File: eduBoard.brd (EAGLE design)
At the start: 101.6 x 80 mm, 31 parts, among them CN1 LED-RGB1, CN2 LED-RGB2, CN3 LED-RGB3

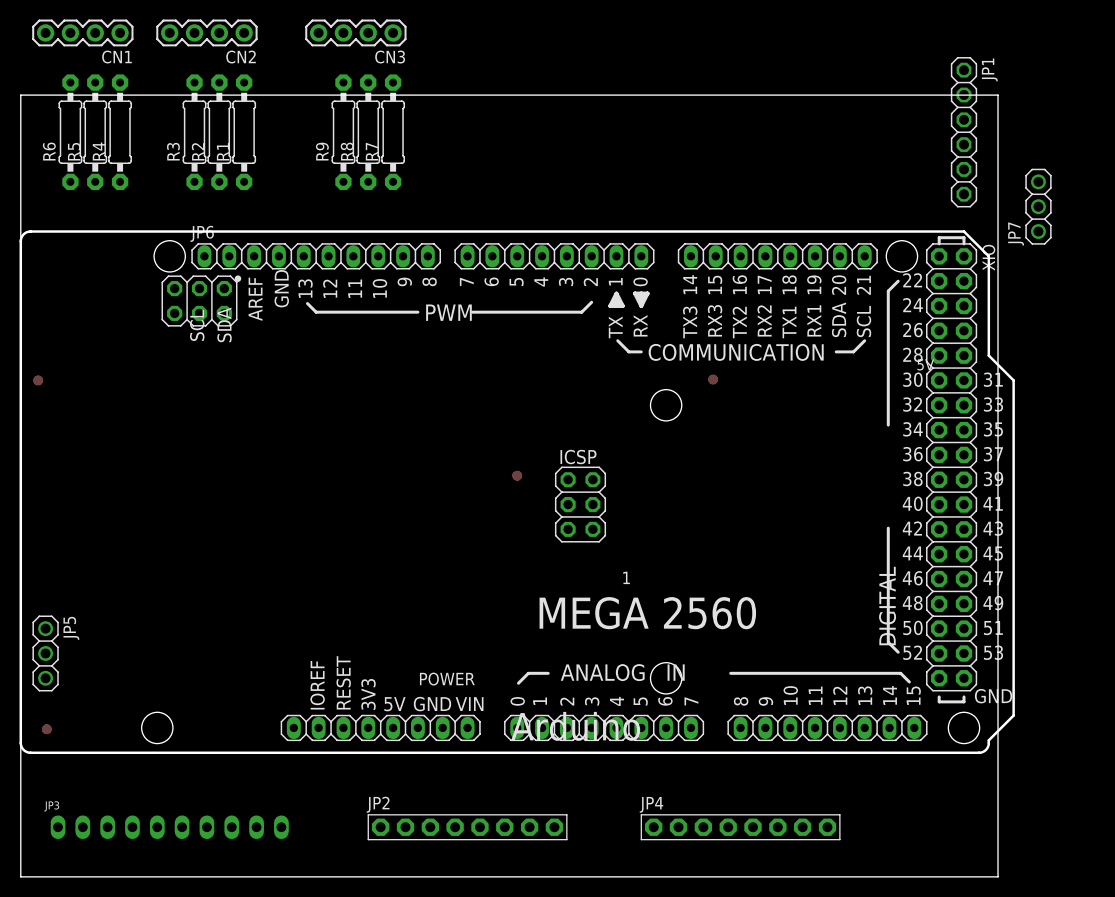
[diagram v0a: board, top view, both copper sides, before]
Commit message: updates, ready for beutification
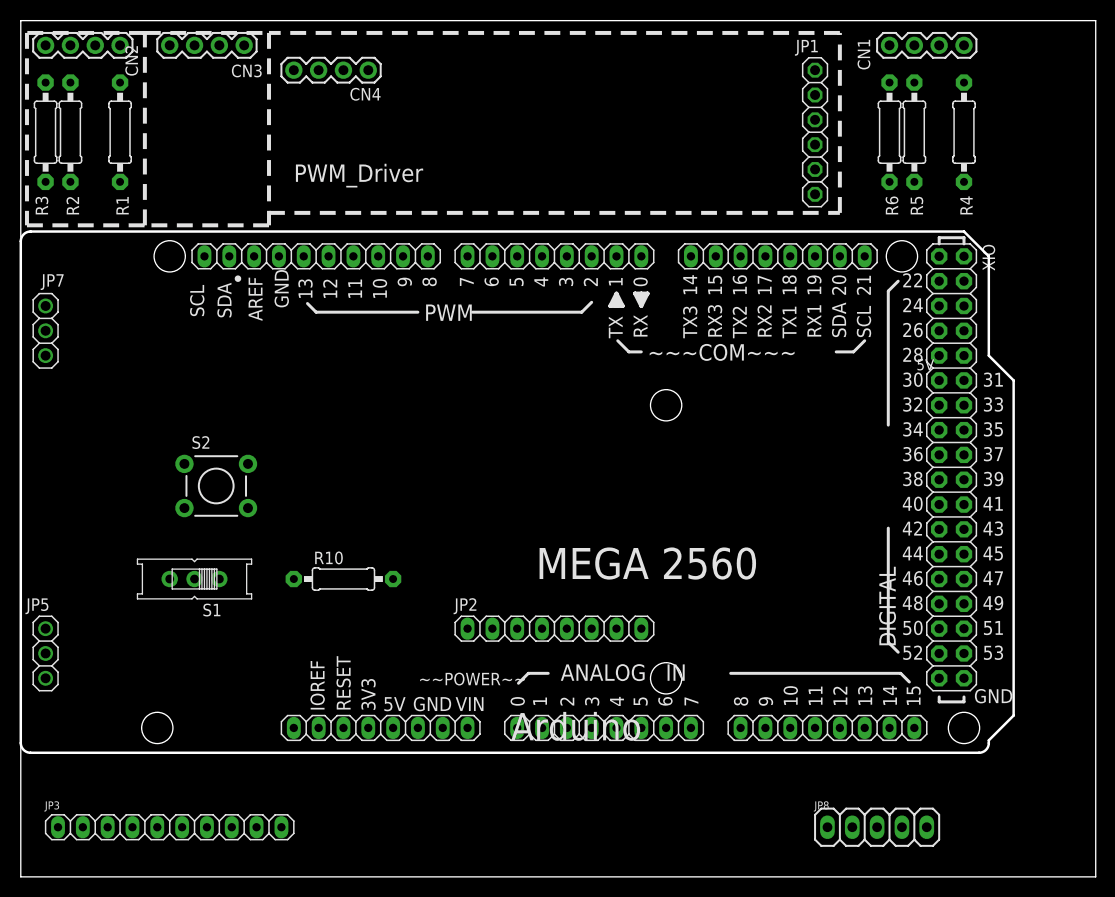
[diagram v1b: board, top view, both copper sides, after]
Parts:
- removed FD1, FD2, FD3, FD4: FIDUCIALMOUNT, SmartPrj:FIDUCIA-MOUNT
- removed ICSP, ICSP1: 3x2M, SmartPrj:2X03
- removed JP4: (no value), adafruit:1X08-BIG
- removed R7, R8, R9: (no value), adafruit:0207/10
- added CN4: PWM-13/16, adafruit:1X04-BIG
- added JP8: (no value), eduBoard:1X05_OVAL
- added R10: (no value), adafruit:0207/10
- added S1: (no value), adafruit:EG1218
- added S2: SWITCH-MOMENTARY-2PTH, eduBoard:TACTILE-PTH
- CN1: value LED-RGB1 -> LED-RGB2
- CN2: value LED-RGB2 -> LED-RGB1
- JP2: device adafruit:1X08-BIG -> eduBoard:1X08-OVAL
- JP3: device microbuilder:1X10_OVAL -> eduBoard:1X10
- moved JP7 102.4 mm to (2.54, 55.9)
- moved CN1 86.4 mm to (96.5, 85.1)
- moved R4 86.4 mm to (96.5, 76.2)
- moved R6 83.8 mm to (88.9, 76.2)
- moved R5 83.8 mm to (91.4, 76.2)
- moved CN3 22.9 mm to (15.2, 85.1), turned to 0 degrees
- moved JP2 20.3 mm to (45.7, 25.4)
- moved R3 15.2 mm to (2.54, 76.2)
- moved R2 15.2 mm to (5.08, 76.2)
- moved JP1 15.2 mm to (81.3, 76.2)
- moved CN2 12.8 mm to (10.2, 85.1)
- moved R1 12.7 mm to (10.2, 76.2)
- renumbered ADCH to ~~~ADC~~~, COMMUNICATION to ~~~COM~~~, POWER to ~~POWER~~, PWML to ~~~PWM~~~
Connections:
- removed net MISO2: ICSP1.1
- removed net MOSI2: ICSP1.4
- removed net N$1: R6.1
- removed net N$11: R4.1
- removed net N$15: R3.1
- removed net N$20: JP2.5
- removed net N$21: R2.1
- removed net N$22: R1.1
- removed net N$24: JP4.1
- removed net N$25: JP4.2
- removed net N$29: JP4.6
- removed net N$30: JP4.7
- removed net N$4: CN3.4, R9.2
- removed net N$45: CN3.1, R7.2
- removed net N$6: R5.1
- removed net N$7: CN3.3, R8.2
- removed net RESET2: ICSP1.5
- removed net SCK2: ICSP1.3
- new net 3V3: JP2.6
- new net IOREF: ~~POWER~~.2
- new net N$13: R10.1, S1.P
- new net PWM13: CN4.1
- new net PWM14: CN3.4, CN4.2
- new net PWM15: CN3.3, CN4.3
- new net PWM16: CN3.1, CN4.4
- net +5V: now also S1.S; no longer ICSP.2, ICSP1.2, JP2.6, ~~POWER~~.2
- net ADC3: now also JP8.2; no longer JP4.8
- net GND: now also S2.1; no longer ICSP.6, ICSP1.6
- net N$10: now also R10.2
- net PA1: now also JP8.1
- net PA7: no longer JP4.3
- net PB1: now also JP2.5; no longer ICSP.3
- net PB2: no longer ICSP.4
- net PB3: no longer ICSP.1
- net PB4: now also R2.1; no longer R8.1
- net PB5: now also R1.1; no longer R7.1
- net PB6: now also R3.1
- net PC4: now also JP8.4; no longer JP4.4
- net PC6: now also JP8.5; no longer JP4.5
- net PC7: now also JP8.3
- net PH6: no longer R9.1
- net PL3: now also R6.1
- net PL4: now also R4.1
- net PL5: now also R5.1
- net RESET: now also S2.3, ~~POWER~~.3; no longer ICSP.5, ~~POWER~~.1
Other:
- board size 101.6 x 80 mm -> 110 x 87.6 mm
- board text added: "PWM_Driver"
